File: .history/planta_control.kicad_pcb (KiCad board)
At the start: 2 copper layers, 80 x 75 mm, 55 parts, among them J1 Conn_01x15_Pin, J2 USB_C_Receptacle, J3 Conn_01x15_Pin, J4 Conn_01x04_Pin, J5 Conn_01x06_Pin, J6 Conn_01x02_Pin, J7 Conn_01x02_Pin, Q1 MMBT3904, Q2 MMBT3904, SW1 SW_DIP_x01, T1 TIP31C, T2 TIP31C, U2 LM358, U3 DS18B20, U4 DS18B20, U5 DS18B20Z, U6 DS18B20Z

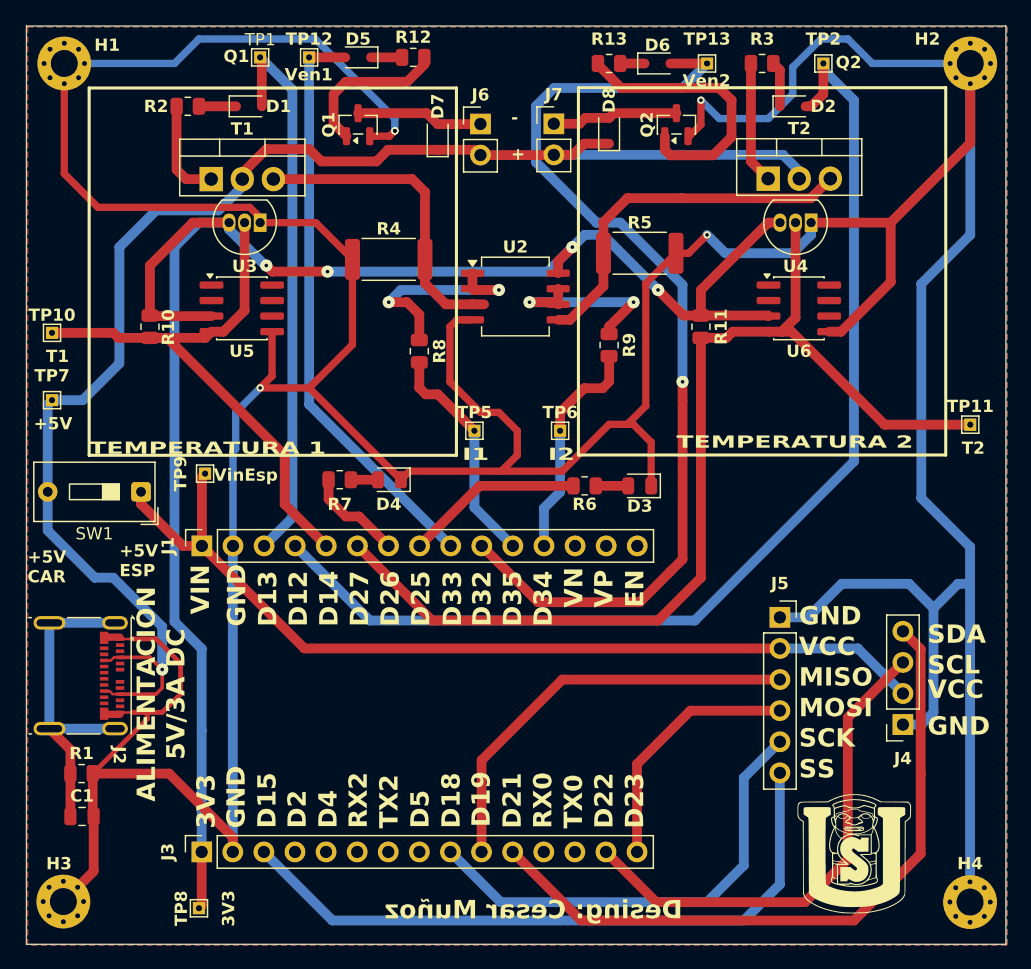
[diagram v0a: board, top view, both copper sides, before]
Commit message: .
.
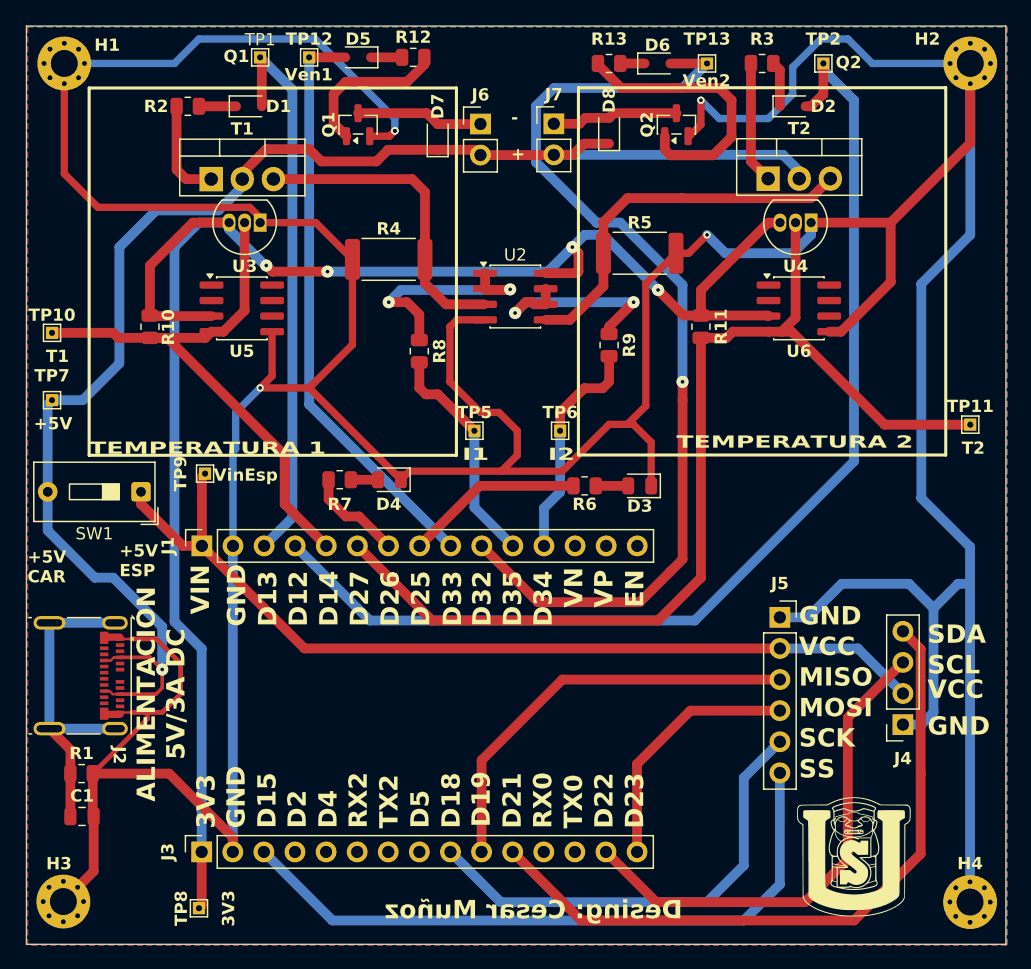
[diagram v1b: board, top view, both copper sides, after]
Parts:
- U2: footprint Package_SO:SOIC-8_5.3x6.2mm_P1.27mm -> Package_SO:SOIC-8_3.9x4.9mm_P1.27mm
- moved G*** 0.25 mm to (92.5, 97.8)
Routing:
- net +3.3V: track 140.8 -> 143.1 mm
- net Net-(U2B--): track 15.6 -> 17.7 mm
- net GND: track 427.5 -> 428.6 mm
- net Net-(U2B-+): track 30.1 -> 31.1 mm
- net Net-(U2A--): track 17.9 -> 18.7 mm

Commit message: .
.
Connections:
- net AT1 renamed AT1/D26
- net AT2 renamed AT2/D25
- net MISO renamed MISO/D19
- net MOSI renamed MOSI/D23
- net Q1 renamed Q1/D13
- net Q2 renamed Q2/D12
- net SCK renamed SCK/D18
- net SCL renamed SCL/D22
- net SDA renamed SDA/D21
- net SS renamed SS/D15
- net T1 renamed T1/D14
- net T2 renamed T2/D27
- net Ven1 renamed Ven1/D33
- net Ven2 renamed Ven2/D32
- net corriente_Q1 renamed corriente_Q1/D35
- net corriente_Q2 renamed corriente_Q2/D34
- net vcc_esp renamed vcc_esp/vin
